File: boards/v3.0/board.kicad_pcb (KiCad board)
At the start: 2 copper layers, 168.3 x 78.7 mm, 66 parts, among them J1 KF301-2P, J2 KF301-2P, J3 KF301-2P, J4 KF301-2P, J5 KF301-2P, J6 KF301-2P, P1 Pin Header, P2 Pin Header, P3 Pin Header, P4 Pin Header, P5 Pin Header, SW1 SS-12D00G 4mm, SW2 SS-12D00G 4mm, T1 ZMPT101B, T2 ZMPT101B, T3 ZMPT101B, U1 TL082, U2 TL082, U3 TL082, U4 TL082, U5 TL082, U6 TL082

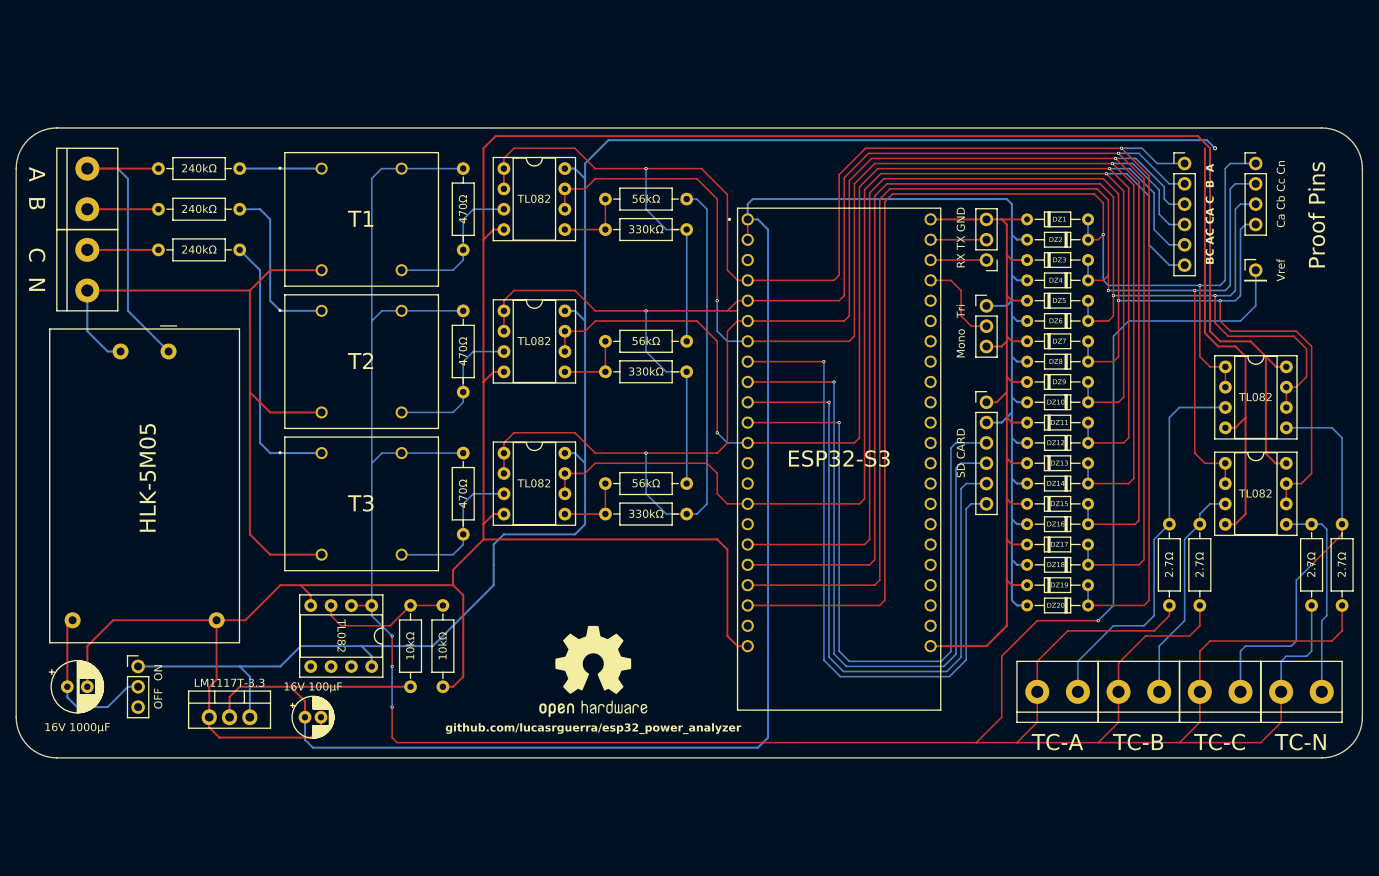
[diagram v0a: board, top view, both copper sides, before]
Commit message: Revision of the v3.0 board
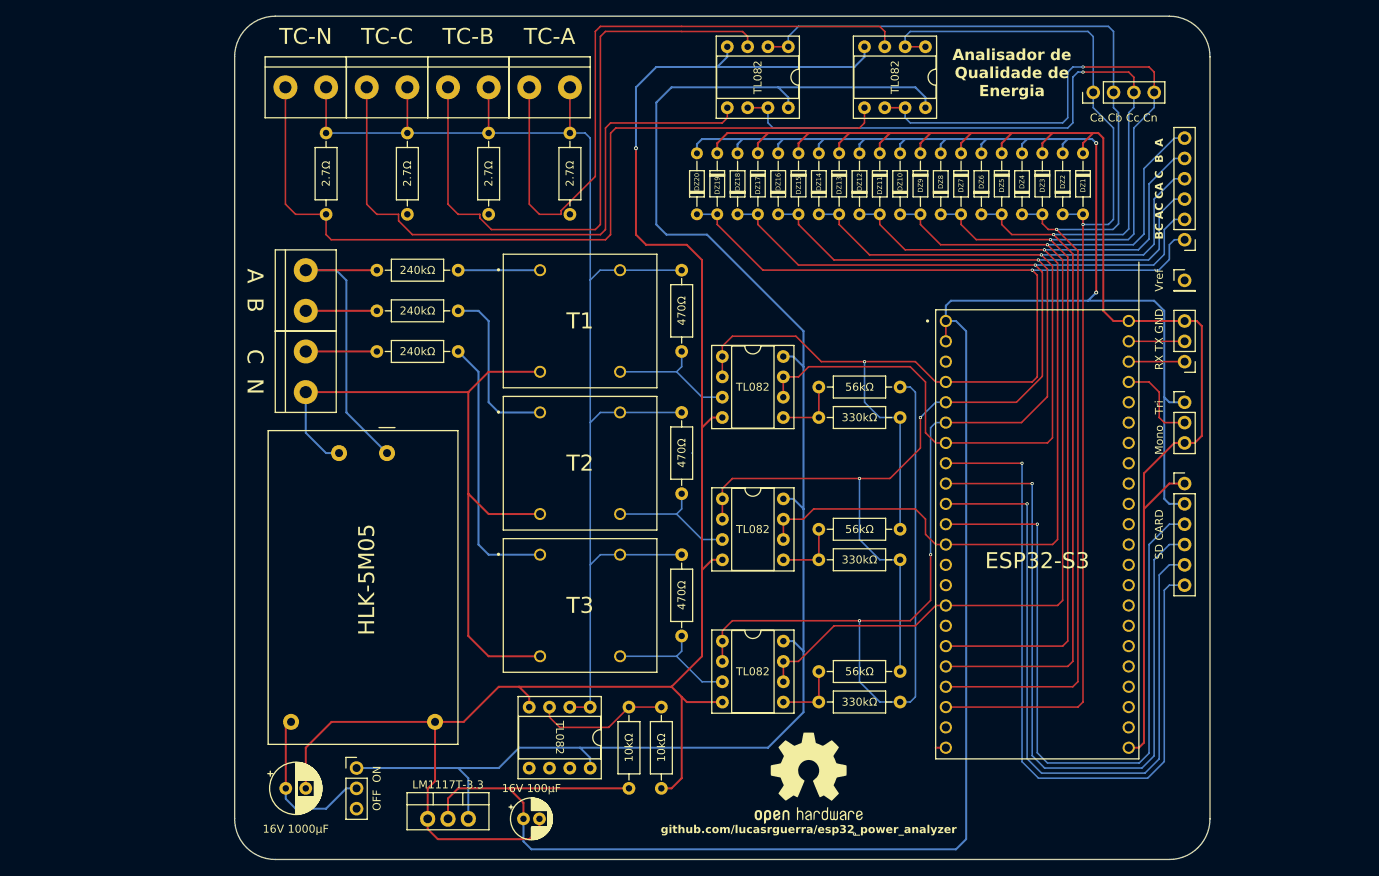
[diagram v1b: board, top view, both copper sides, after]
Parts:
- moved J6 141.3 mm to (102.2, 44.5), turned to 180 degrees
- moved R18 129.1 mm to (102.2, 60.3), turned to 90 degrees
- moved J5 124.6 mm to (112.4, 44.5), turned to 180 degrees
- moved R17 123.1 mm to (112.4, 60.3), turned to 90 degrees
- moved J4 109.1 mm to (122.6, 44.5), turned to 180 degrees
- moved R16 97.0 mm to (122.6, 60.3), turned to 90 degrees
- moved J3 95.5 mm to (132.7, 44.5), turned to 180 degrees
- moved R15 84.3 mm to (132.7, 60.3), turned to 90 degrees
- moved DZ20 69.2 mm to (148.6, 60.3), turned to 90 degrees
- moved U5 67.7 mm to (160.0, 39.4), turned to -90 degrees
- moved DZ19 66.4 mm to (151.1, 52.7), turned to -90 degrees
- moved U6 64.2 mm to (177.2, 39.4), turned to -90 degrees
- moved DZ18 62.0 mm to (153.7, 60.3), turned to 90 degrees
- moved DZ17 59.4 mm to (156.2, 52.7), turned to -90 degrees
- moved DZ16 54.8 mm to (158.8, 60.3), turned to 90 degrees
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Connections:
- R15 pad 1: TC A-1 -> TC B-1
- R16 pad 1: TC B-1 -> TC C-1
- R17 pad 1: TC C-1 -> TC A-1
- U5 pad 1: Current A -> Current B
- U5 pad 2: Current A -> Current B
- U5 pad 3: TC A-1 -> TC B-1
- U6 pad 1: Current B -> Current A
- U6 pad 2: Current B -> Current A
- U6 pad 3: TC B-1 -> TC A-1
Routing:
- net TC A-2: track 417.1 -> 165.7 mm, vias 4 -> 0
- net TC N-1: track 25.9 -> 105.7 mm
- net Treated Wave A: track 210.3 -> 151.5 mm
- net Vin: track 260.2 -> 204.0 mm, vias 1 -> 0
- net GND: track 464.5 -> 411.8 mm, vias 0 -> 1
- net TC B-1: track 28.0 -> 79.2 mm
- net Treated Wave CA: track 172.9 -> 123.9 mm, vias 2 -> 1
- net Treated Wave AB: track 175.3 -> 129.5 mm, vias 2 -> 1
- net Treated Wave B: track 197.2 -> 157.3 mm, vias 2 -> 3
- net Treated Wave C: track 236.8 -> 202.6 mm, vias 2 -> 3
- net Treated Wave BC: track 168.2 -> 134.1 mm
- net TC A-1: track 48.8 -> 82.4 mm
- net Vcc: track 274.8 -> 307.6 mm, vias 0 -> 2
- net TC C-1: track 47.8 -> 76.5 mm, vias 1 -> 0
- net Current N: track 181.7 -> 156.0 mm
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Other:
- board size 168.3 x 78.7 mm -> 121.9 x 105.4 mm
- board text added: "Analisador de Qualidade de Energia"
- board text removed: "Proof Pins"
